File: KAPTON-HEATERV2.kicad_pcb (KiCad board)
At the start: 2 copper layers, 97.8 x 82.2 mm, 16 parts, among them J1 XT60PW-M, J2 XT60PW-M, J3 Screw_Terminal_01x10, J4 Screw_Terminal_01x04, J5 10090926-P154XLF, K1 1-1393210-8

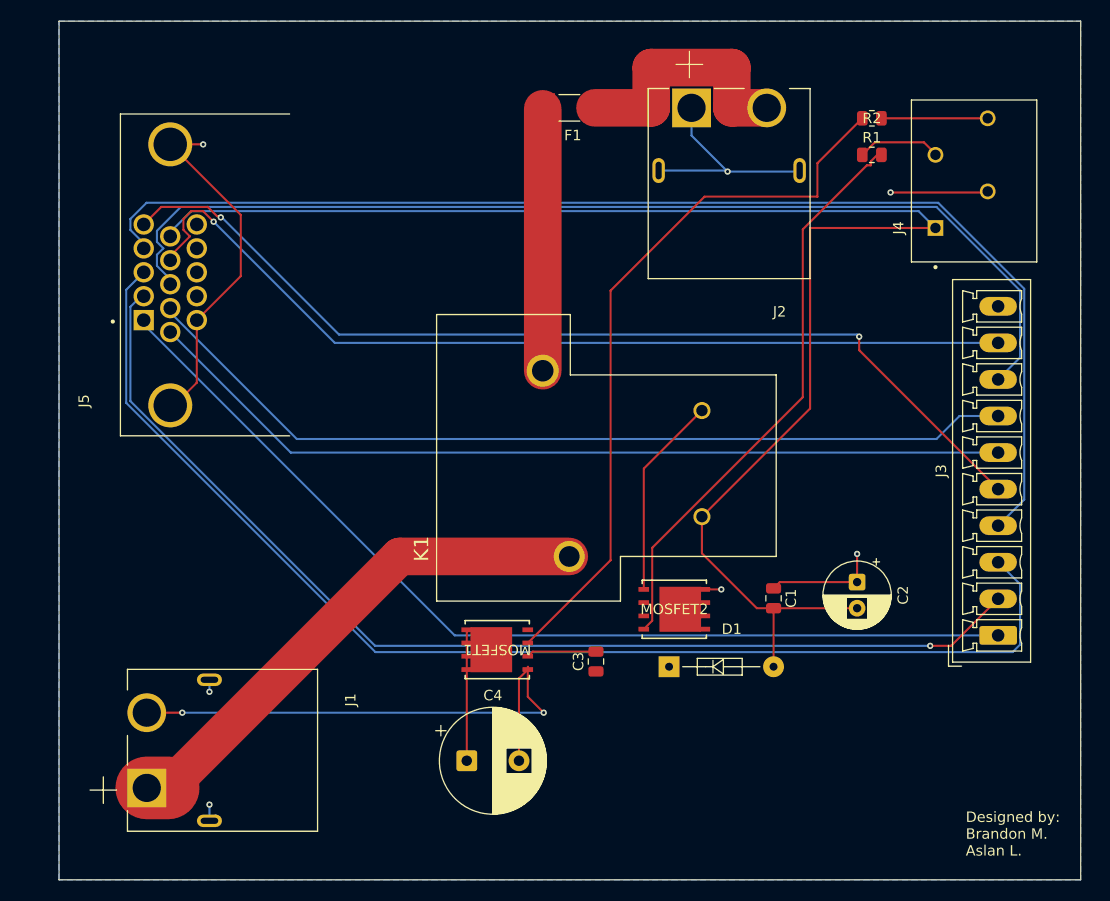
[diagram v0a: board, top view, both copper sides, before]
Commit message: Done?
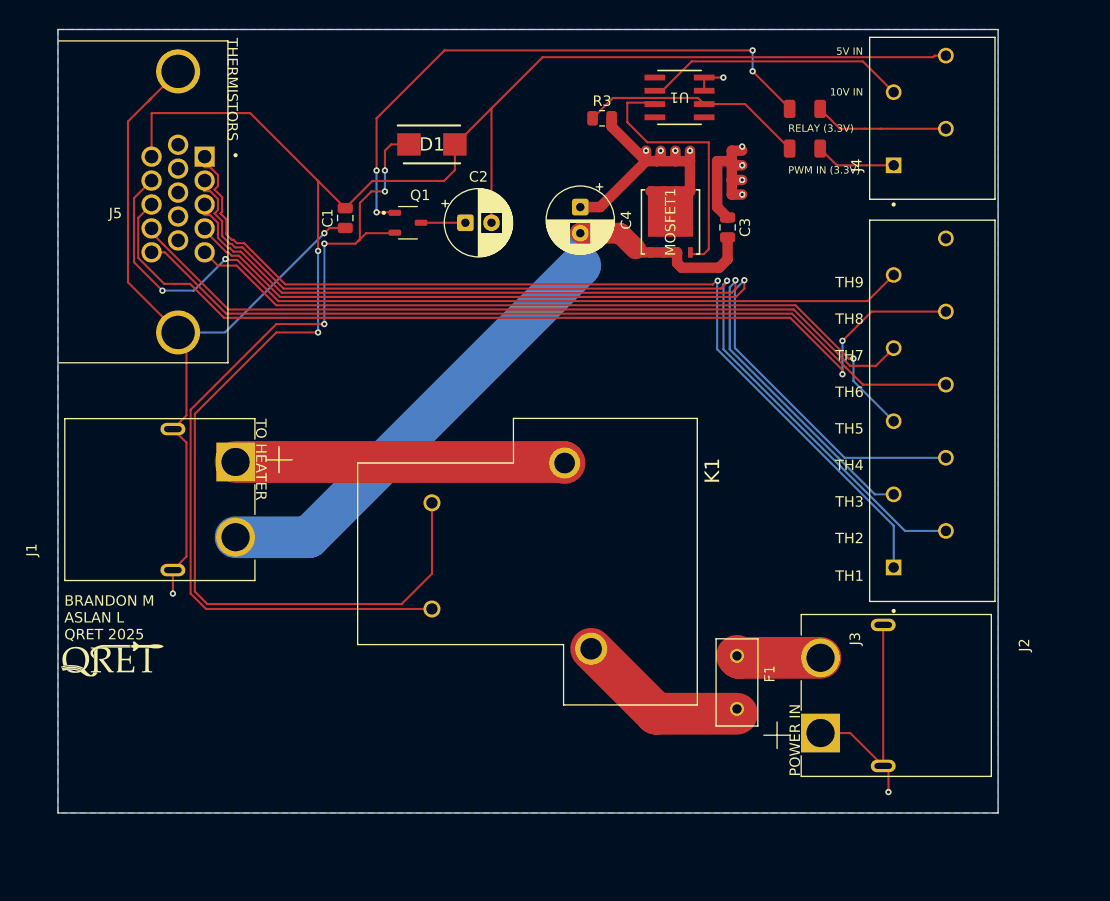
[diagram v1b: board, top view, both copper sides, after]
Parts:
- removed MOSFET2: SIR462DP-T1-GE3, SIR462DP:POWERPAK_SO-8_SINGLE_VIS
- added G***: LOGO, LOGO, F.Cu at (29.7, 100.2)
- added Q1: AO3400A, AO3400A (1):SOT95P280X125-3N, F.Cu at (58.0, 58.5)
- added R3: R100k, Resistor_SMD:R_0805_2012Metric, F.Cu at (76.6, 48.5)
- added U1: TC4427ACOA, TC4427:SOIC8-N_MC_MCH, F.Cu at (84.0, 46.5)
- C4: value C1000uf -> C10uf; footprint Capacitor_THT:CP_Radial_D10.0mm_P5.00mm -> Capacitor_THT:CP_Radial_D6.3mm_P2.50mm
- D1: value 1N4148 -> MBRS1100T3G; footprint digikey-footprints:Diode_DO-35_P10mm -> MBRS1100T3G:DIOM5436X247N
- F1: value 0679L9200-01 -> 20A Fuse; footprint 0679L9200_01:FUSC6125X279N -> FUSE_0697H9200:FUSRR508W60L835T400H810
- J3: value Screw_Terminal_01x10 -> 1985276; footprint Connector_Phoenix_MC:PhoenixContact_MCV_1,5_10-G-3.5_1x10_P3.50mm_Vertical -> 01x12 connnector:PHOENIX_1985276
- J4: value Screw_Terminal_01x04 -> 1985218
- R1, R2: footprint Resistor_SMD:R_0805_2012Metric -> PCM_JLCPCB:R_1206
- moved F1 57.3 mm to (89.5, 102.5), turned to -90 degrees
- moved D1 54.9 mm to (60.3, 51.0)
- moved C1 54.8 mm to (52.0, 58.0), turned to 90 degrees
- moved C4 54.1 mm to (74.5, 57.0), turned to -90 degrees
- moved J2 52.4 mm to (103.5, 103.8), turned to -90 degrees
- moved C2 50.9 mm to (63.5, 58.5), turned to 0 degrees
- moved MOSFET1 44.2 mm to (83.1, 58.4), turned to 90 degrees
- moved C3 43.4 mm to (88.6, 59.0), turned to -90 degrees
- moved J1 24.3 mm to (35.5, 85.0), turned to 90 degrees
- moved K1 12.5 mm to (69.4, 90.9), turned to -90 degrees
- moved R1 7.78 mm to (96.0, 47.6), turned to 180 degrees
- moved J4 7.21 mm to (108.2, 48.5)
- moved R2 7.04 mm to (96.0, 51.4)
- moved J5 7.03 mm to (36.0, 56.5), turned to -90 degrees
- moved J3 3.26 mm to (114.2, 94.8)
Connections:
- net Net-(F1-Pad2) renamed /24VIN2
- J4 pad 1: 5V -> PWM
- J4 pad 2: GND -> RELAY
- J4 pad 3: RELAY -> 10V
- J4 pad 4: PWM -> 5V
- J5 pad 10: 5V -> unconnected-(J5-Pad10)
- J5 pad 11: GND -> 5V
- J5 pad 12: unconnected-(J5-Pad12) -> TH9
- J5 pad 13: unconnected-(J5-Pad13) -> TH8
- J5 pad 14: unconnected-(J5-Pad14) -> TH7
- J5 pad 15: unconnected-(J5-Pad15) -> TH6
- J5 pad 6: TH6 -> unconnected-(J5-Pad6)
- J5 pad 7: TH7 -> unconnected-(J5-Pad7)
- J5 pad 8: TH8 -> unconnected-(J5-Pad8)
- J5 pad 9: TH9 -> unconnected-(J5-Pad9)
- MOSFET1 pad 3: Net-(MOSFET1-Pad3) -> Net-(J1-Pin_2)
- MOSFET1 pad 4: Net-(J1-Pin_2) -> 10V PWM
- R2 pad 2: Net-(MOSFET1-Pad3) -> Net-(U1-INPUT_A)
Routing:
- net Net-(MOSFET1-Pad3): track 69.8 -> 0.00 mm
- net Net-(D1-K): track 19.4 -> 85.7 mm, vias 0 -> 4
- net GND: track 91.0 -> 152.0 mm, vias 5 -> 12
- net 5V: track 145.5 -> 180.2 mm, vias 0 -> 2
- net TH3: track 117.7 -> 85.1 mm, vias 0 -> 1
- net TH4: track 117.8 -> 87.1 mm, vias 0 -> 1
- net 10V PWM: track 0.00 -> 25.4 mm
- net 10V: track 0.00 -> 25.3 mm
- net Net-(U1-INPUT_A): track 0.00 -> 21.7 mm
- net TH5: track 94.5 -> 73.9 mm, vias 2 -> 1
- net /24V: track 49.8 -> 31.5 mm
- net /24VIN: track 25.3 -> 8.08 mm
- net TH2: track 105.4 -> 92.6 mm
- net TH8: track 102.4 -> 92.2 mm, vias 0 -> 2
- net /24VIN2: track 25.8 -> 17.0 mm
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- added copper zone on B.Cu, net GND
- removed copper zone on B.Cu, net (none)
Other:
- board size 97.8 x 82.2 mm -> 90 x 75 mm
- board text added: "10V IN"
- board text added: "5V IN"
- board text added: "BRANDON M ASLAN L QRET 2025"
- board text added: "POWER IN"
- board text added: "PWM IN (3.3V)"
- board text added: "RELAY (3.3V)"
- board text added: "TH1"
- board text added: "TH2"
- board text added: "TH3"
- board text added: "TH4"
- board text added: "TH5"
- board text added: "TH6"
- board text added: "TH7"
- board text added: "TH8"
- board text added: "TH9"
- board text added: "THERMISTORS"
- board text added: "TO HEATER"
- board text removed: "Designed by: Brandon M. Aslan L."
